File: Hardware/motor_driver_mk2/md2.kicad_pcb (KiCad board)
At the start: 2 copper layers, 43.2 x 88.3 mm, 17 parts, among them J1 mode&en M1, J10 mode&en M1, J11 mode&en M2, J12 M1, J13 M2, J14 mode&en M2, J2 M1, J3 Logic supply voltage, J4 Power supply voltage, J5 M2, J6 mode&en M2, J7 mode&en M1, J8 M1, J9 M2, U1 L293D, U2 L293D, U3 L293D

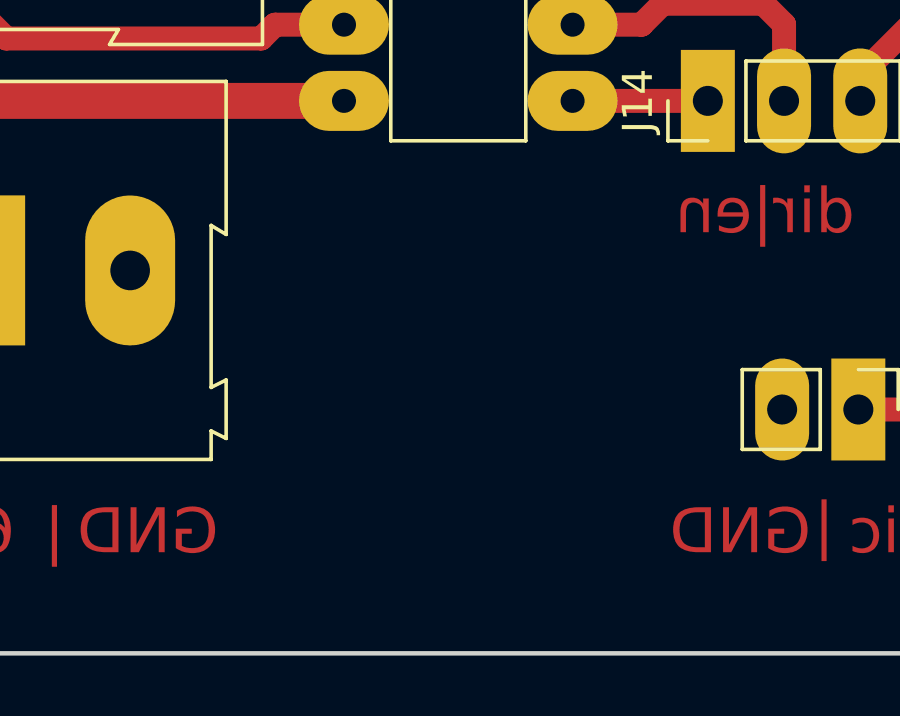
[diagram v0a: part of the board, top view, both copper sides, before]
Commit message: ponerla wapa
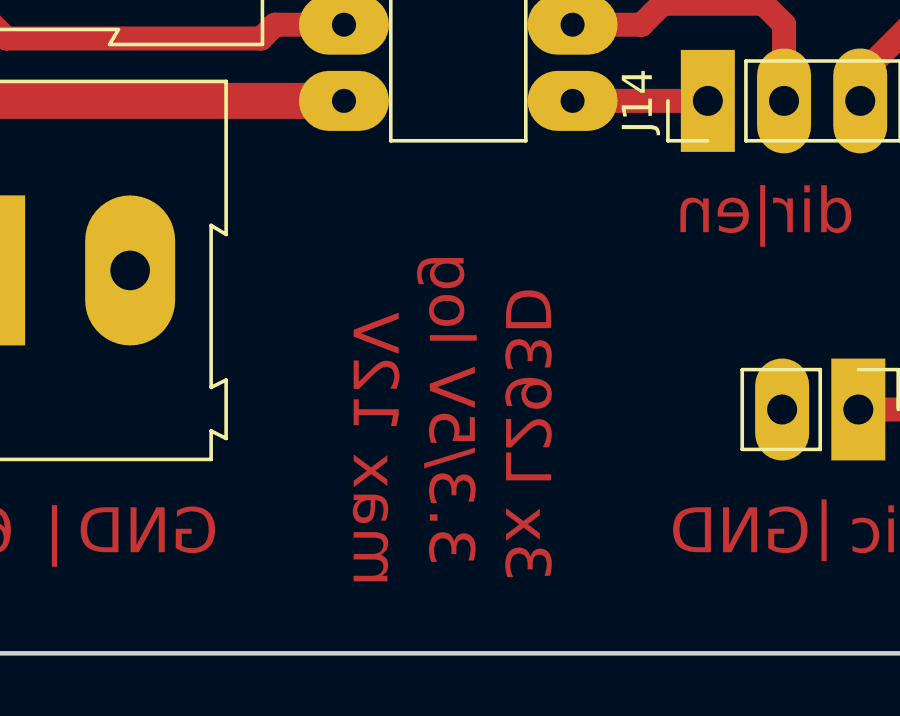
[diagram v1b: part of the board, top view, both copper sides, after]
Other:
- board text added: "3.3/5V log"
- board text added: "3x L293D"
- board text added: "max 12V"
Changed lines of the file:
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@@
 (kicad_pcb (version 4) (host pcbnew 4.0.7-e2-6376~58~ubuntu16.04.1)
   (general
-    (links 50)
-    (no_connects 14)
+    (links 0)
+    (no_connects 1)
     (area 155.856 52.0365 204.656572 143.707)
     (thickness 1.6)
-    (drawings 17)
+    (drawings 20)
     (tracks 128)
     (zones 0)
@@
     )
   )
+  (gr_text "max 12V" (at 175.514 134.1755 270) (layer F.Cu)
+    (effects (font (size 1.5 1.5) (thickness 0.3)) (justify mirror))
+  )
+  (gr_text "3.3/5V log" (at 178.054 132.842 270) (layer F.Cu)
+    (effects (font (size 1.5 1.5) (thickness 0.3)) (justify mirror))
+  )
+  (gr_text "3x L293D" (at 180.594 133.6675 270) (layer F.Cu)
+    (effects (font (size 1.5 1.5) (thickness 0.3)) (justify mirror))
+  )
   (gr_text | (at 190.5 136.7155) (layer F.Cu)
